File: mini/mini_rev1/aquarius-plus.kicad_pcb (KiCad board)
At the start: 2 copper layers, 128 x 83 mm, 109 parts, among them J1 Power in, J10 FPGA spare, J13 ESP32 spare, J2 ESP USB Host, J3 Audio out, J4 VGA, J9 TF-03A, Q3 2N7002, SW1 SW_DPDT_x2, U10 ESP32-S3-WROOM-1-N4R2, U11 LDL1117S33R, U13 IS61C5128AL-10TLI, U3 LD1117S12, U6 XC6SLX9-2TQG144C, X1 SX3M14.31818M20F30TNN

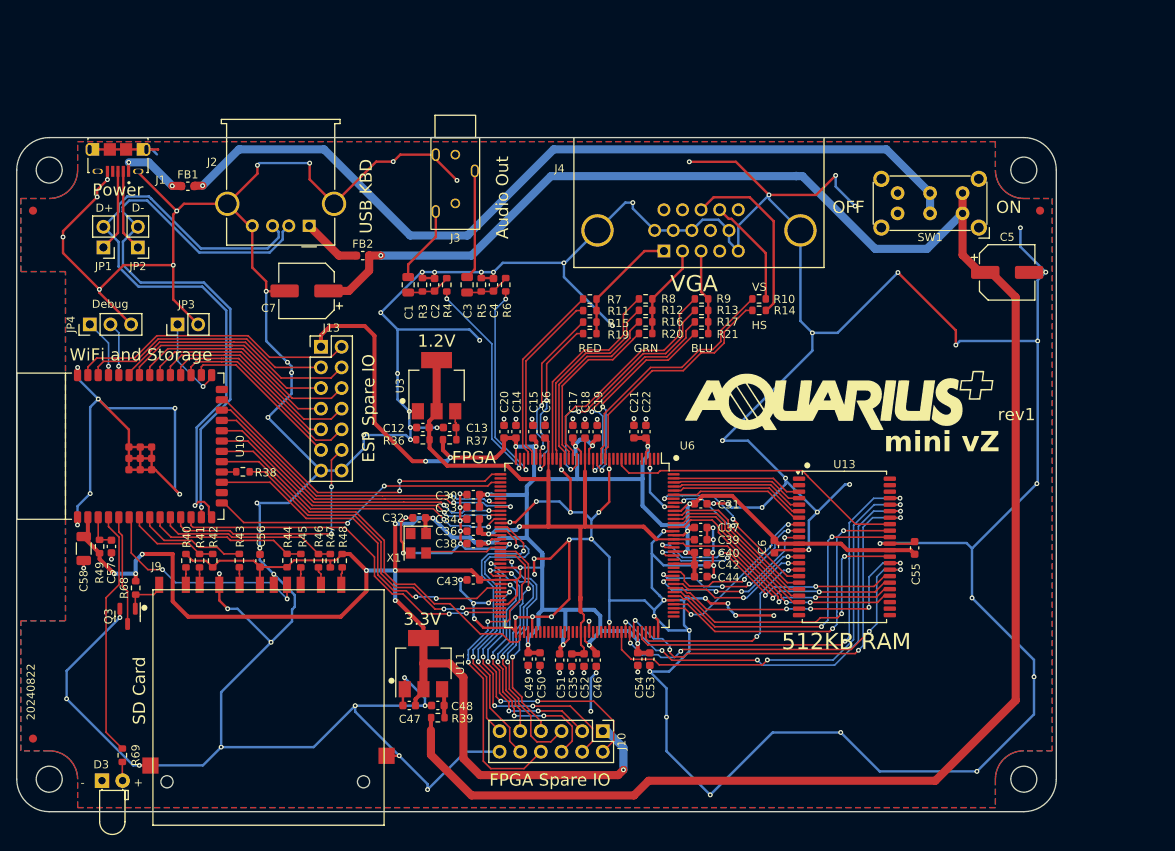
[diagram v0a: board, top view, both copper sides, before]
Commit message: Mini vZ rev1
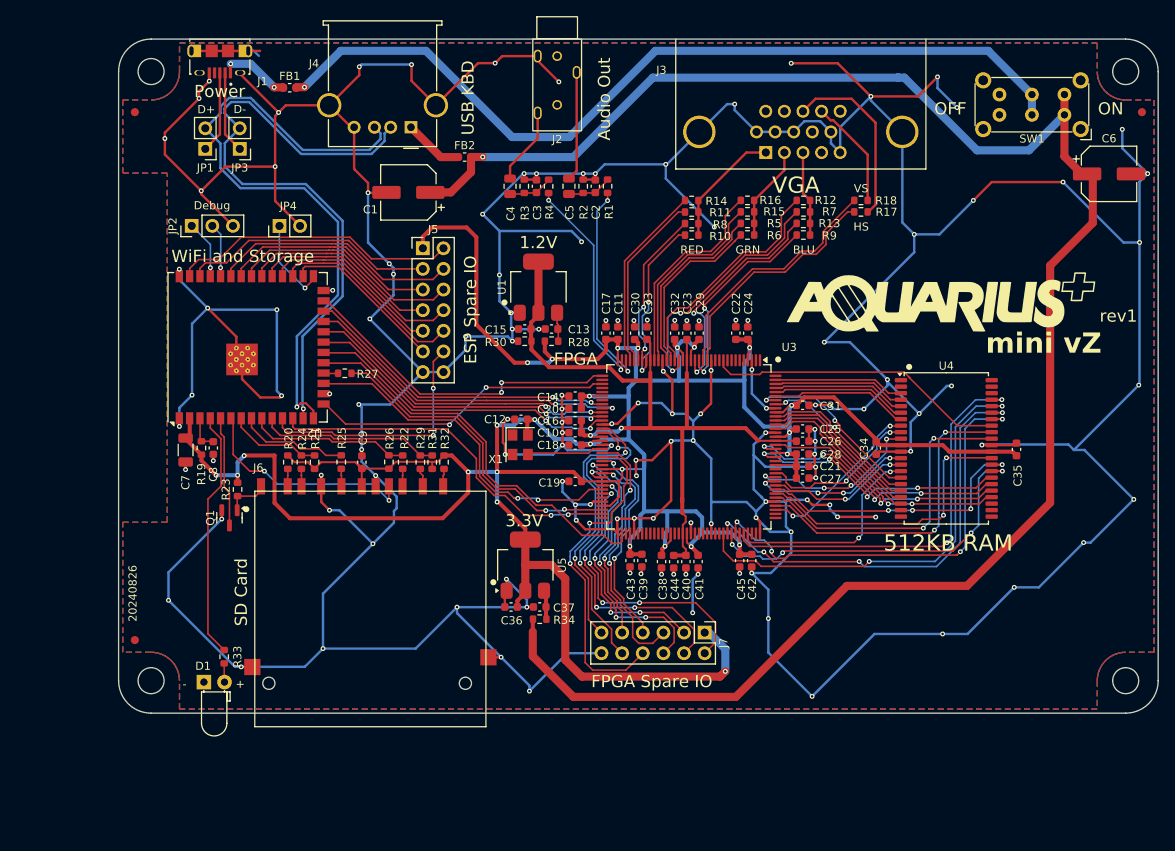
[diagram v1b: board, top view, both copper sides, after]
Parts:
- U2: renamed from U10; footprint aquarius-plus:ESP32-S2-SOLO-N4R2 -> RF_Module:ESP32-S3-WROOM-1U
- moved U2 30.9 mm to (93.4, 68.8)
- moved R17 17.4 mm to (168.9, 52.1)
- moved #G1 17.4 mm to (178.8, 63.2)
- moved R13 17.4 mm to (161.9, 53.6)
- moved U1 17.4 mm to (129.2, 61.4)
- moved C15 17.4 mm to (127.5, 66.6)
- moved C16 17.4 mm to (133.7, 77.9)
- moved FB1 17.4 mm to (98.6, 36.9)
- moved J5 17.4 mm to (115.0, 56.6)
- moved JP4 17.4 mm to (97.3, 53.9)
- moved R1 17.4 mm to (137.7, 49.0)
- moved R27 17.4 mm to (105.4, 72.0)
- moved R30 17.4 mm to (127.5, 68.1)
- moved R32 17.4 mm to (117.6, 83.0)
- moved JP3 17.4 mm to (92.5, 44.4)
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- renumbered C7 to C1, C36 to C10, C14 to C11, C32 to C12, C30 to C14, C12 to C15, C34 to C16, C20 to C17, C38 to C18, C43 to C19, C4 to C2, C33 to C20, C42 to C21, C21 to C22, C18 to C23, C22 to C24, C37 to C25, C39 to C26, C44 to C27, C40 to C28, C19 to C29, C2 to C3, C15 to C30, C17 to C32, C16 to C33, C6 to C34, C55 to C35, C47 to C36, C48 to C37, C51 to C38, C50 to C39, C1 to C4, C52 to C40, C46 to C41, C53 to C42, C49 to C43, C35 to C44, C54 to C45, C3 to C5, C5 to C6, C58 to C7, C57 to C8, C56 to C9, D3 to D1, J3 to J2, J4 to J3, J2 to J4, J13 to J5, J9 to J6, J10 to J7, JP4 to JP2, JP2 to JP3, JP3 to JP4, Q3 to Q1, R6 to R1, R19 to R10, R9 to R12, R17 to R13, R7 to R14, R12 to R15, R8 to R16, R14 to R17, R10 to R18, R49 to R19, R5 to R2, R40 to R20, R42 to R21, R45 to R22, R68 to R23, R41 to R24, R43 to R25, R44 to R26, R38 to R27, R37 to R28, R46 to R29, R36 to R30, R47 to R31, R48 to R32, R69 to R33, R39 to R34, R16 to R5, R20 to R6, R13 to R7, R15 to R8, R21 to R9, U3 to U1, U6 to U3, U13 to U4, U11 to U5
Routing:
- net +5V: track 238.7 -> 224.1 mm
- net GND: track 1031.4 -> 1033.9 mm
- net unconnected-(U2-IO45-Pad26): track 0.00 -> 1.14 mm, vias 0 -> 1
- net ESP_USB_D-: track 76.7 -> 77.7 mm
- net ESP_USB_D+: track 78.9 -> 79.9 mm
- net unconnected-(U2-IO46/I-Pad16): track 0.00 -> 0.76 mm, vias 0 -> 1
- net ESP_EXP2: track 30.1 -> 30.7 mm
- net Net-(JP4-A): track 10.3 -> 10.8 mm
- net ESP_RTS: track 38.1 -> 38.7 mm
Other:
- board text added: "0"
- board text added: "0 mm"
- board text added: "0.01 mm"
- board text added: "0.02"
- board text added: "0.035 mm"
- board text added: "0.2000 mm / 0.0000 mm"
- board text added: "0.3000 mm"
- board text added: "1"
- board text added: "1.51 mm"
- board text added: "1.6000 mm"
- board text added: "128.0000 mm x 83.0000 mm"
- board text added: "2"
- board text added: "20240826"
- board text added: "3.3"
- board text added: "4.5"
- board text added: "B.Cu"
- board text added: "B.Mask"
- board text added: "B.Paste"
- board text added: "B.Silkscreen"
- board text added: "BOARD CHARACTERISTICS"
- board text added: "Blue"
- board text added: "Board Thickness:"
- board text added: "Board overall dimensions:"
- board text added: "Bottom Silk Screen"
- board text added: "Bottom Solder Mask"
- board text added: "Bottom Solder Paste"
- board text added: "Castellated pads:"
- board text added: "Color"
- board text added: "Copper Finish:"
- board text added: "Copper Layer Count:"
- board text added: "Dielectric 1"
- board text added: "Direct Printing"
- board text added: "Edge card connectors:"
- board text added: "Epoxy"
- board text added: "Epsilon R"
- board text added: "F.Cu"
- board text added: "F.Mask"
- board text added: "F.Paste"
- board text added: "F.Silkscreen"
- board text added: "FR4"
- board text added: "HAL lead-free"
- board text added: "Impedance Control:"
- board text added: "Layer Name"
- board text added: "Loss Tangent"
- board text added: "Material"
- board text added: "Min hole diameter:"
- board text added: "Min track/spacing:"
- board text added: "No"
- board text added: "Not specified"
- board text added: "Plated Board Edge:"
- board text added: "Thickness (mm)"
- board text added: "Top Silk Screen"
- board text added: "Top Solder Mask"
- board text added: "Top Solder Paste"
- board text added: "Type"
- board text added: "White"
- board text added: "copper"
- board text added: "core"
- board text removed: "20240822"
